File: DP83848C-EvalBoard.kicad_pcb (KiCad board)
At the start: 4 copper layers, 165 parts, among them J1 Conn_02x08_Odd_Even, J10 RJ45_LED_Shielded, J11 USB_C_Receptacle_USB2.0, J12 Conn_02x05_Odd_Even, J2 Conn_02x08_Odd_Even, J3 Conn_02x04_Odd_Even, J4 Conn_01x04, J5 Conn_01x04, J6 Conn_02x04_Odd_Even, J7 Conn_02x04_Odd_Even, J8 Conn_02x04_Odd_Even, J9 Conn_01x02, Q1 AO3401A, Q2 AO3400A, Q3 AO3401A, SW1 SW_Push, T1 H1102NL, U1 AMS1117-3.3, U2 DP83848C, U3 STM32F407VGTx, U4 USBLC6-2SC6, X1 50MHz, Y1 25MHz

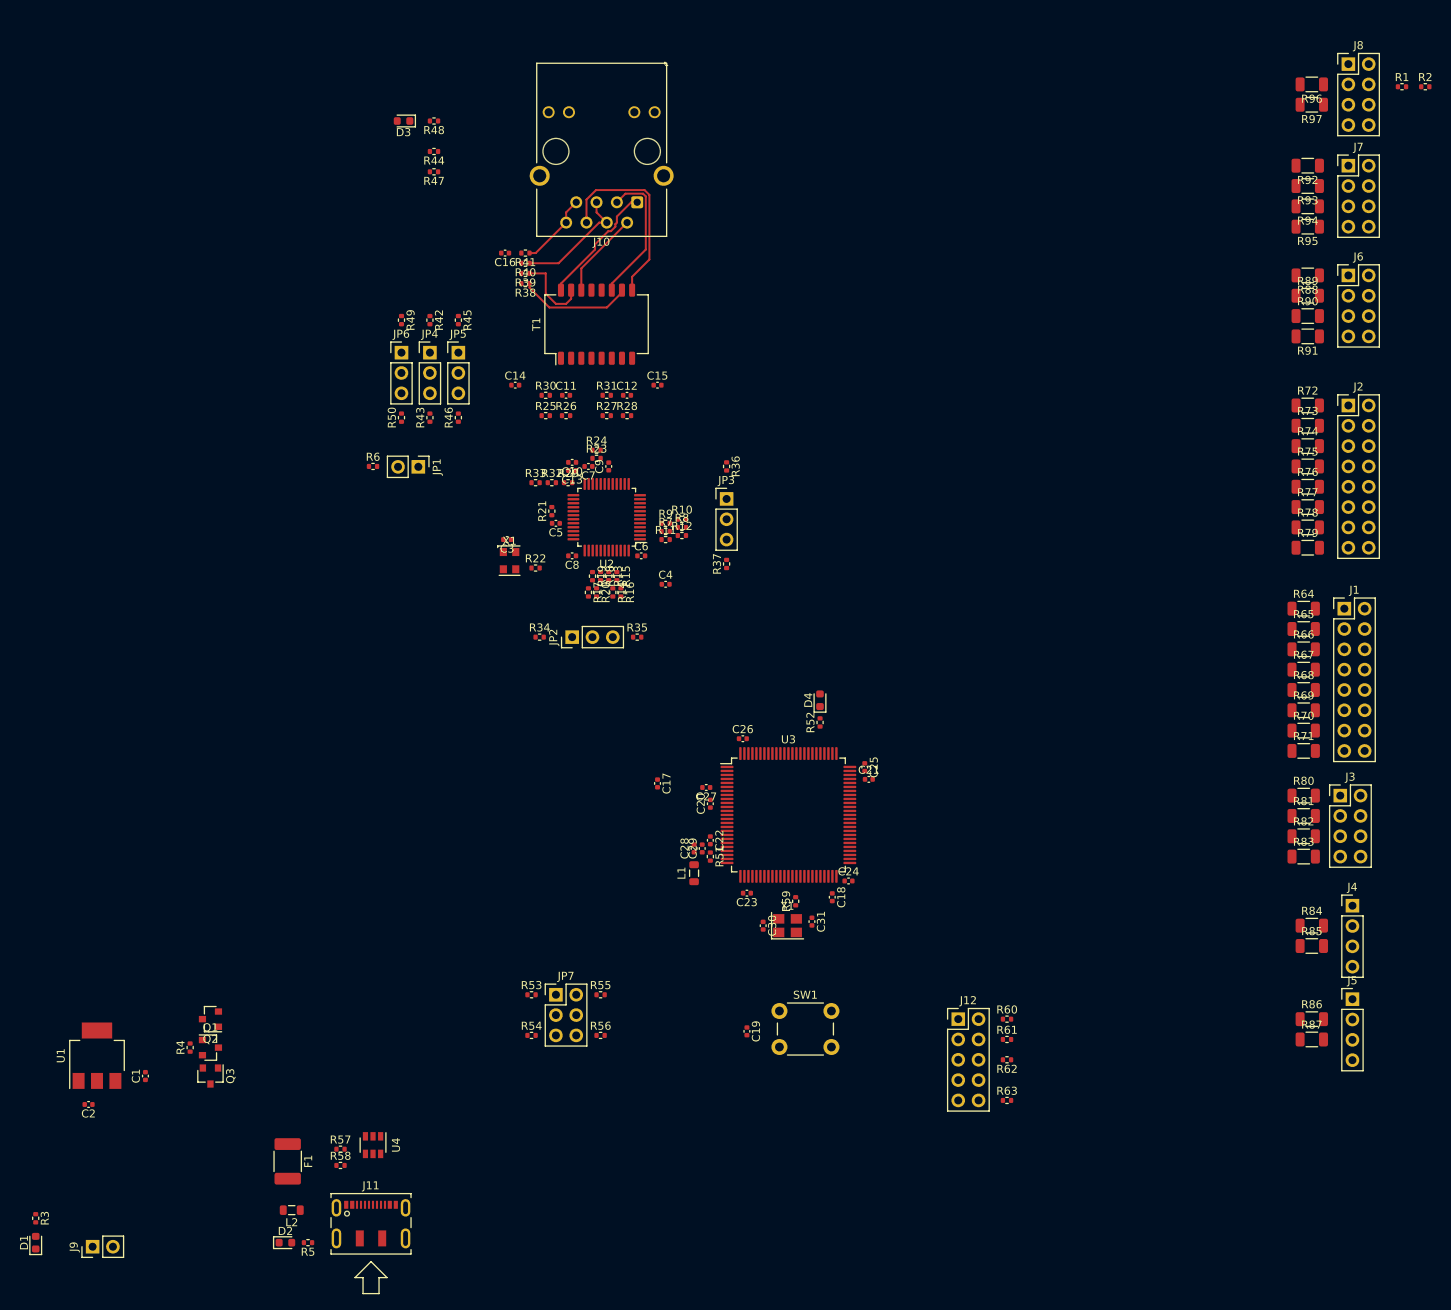
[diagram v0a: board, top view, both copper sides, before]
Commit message: Test...
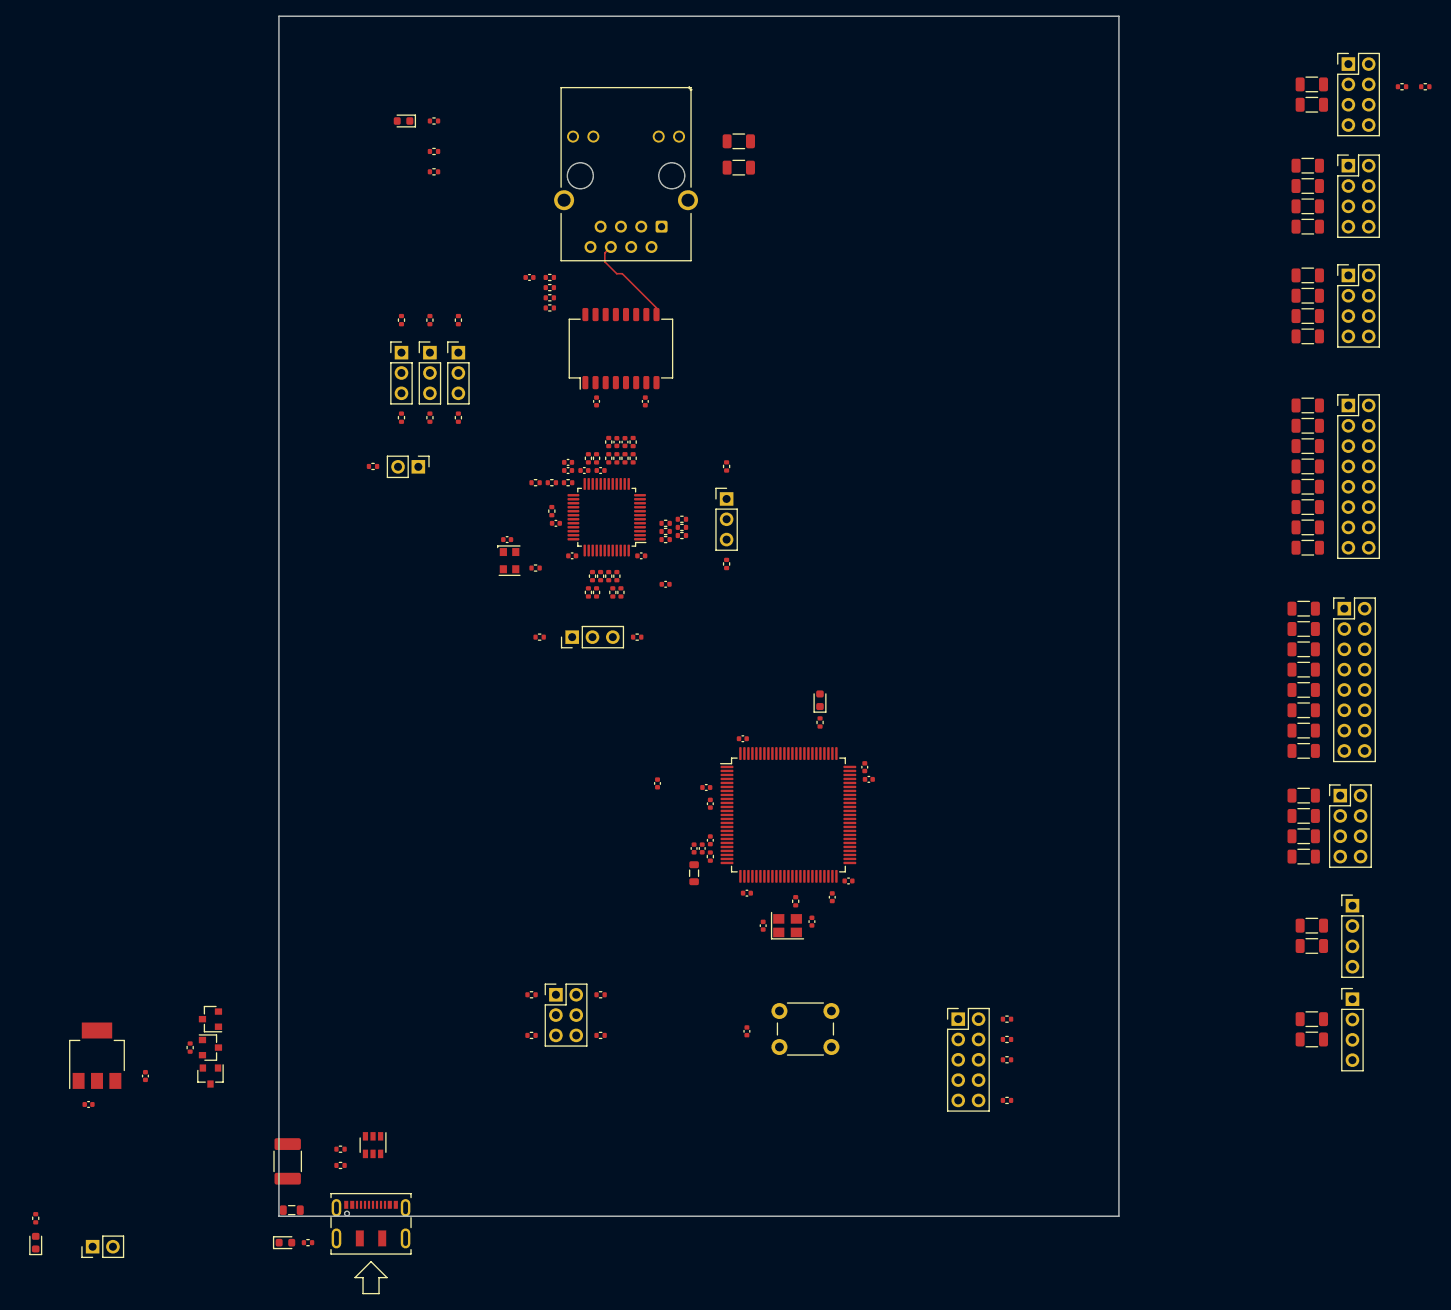
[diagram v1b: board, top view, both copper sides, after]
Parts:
- added R98: 0, Resistor_SMD:R_1206_3216Metric, F.Cu at (157.5, 40.6)
- added R99: 0, Resistor_SMD:R_1206_3216Metric, F.Cu at (157.5, 43.9)
- moved C14 10.4 mm to (139.7, 73.2), turned to 270 degrees
- moved R30 9.80 mm to (141.2, 78.2), turned to 270 degrees
- moved R25 9.51 mm to (141.2, 80.3), turned to 90 degrees
- moved C11 8.63 mm to (142.2, 78.2), turned to 90 degrees
- moved R26 8.29 mm to (142.2, 80.3), turned to 270 degrees
- moved R31 6.71 mm to (144.3, 78.2), turned to 270 degrees
- moved C12 5.85 mm to (143.3, 78.2), turned to 90 degrees
- moved R27 5.80 mm to (143.3, 80.3), turned to 90 degrees
- moved R28 5.39 mm to (144.3, 80.3), turned to 270 degrees
- moved C16 4.31 mm to (131.3, 57.7)
- moved J10 4.31 mm to (147.8, 51.3)
- moved R38 4.31 mm to (133.9, 61.5)
- moved R39 4.31 mm to (133.9, 60.2)
- moved R41 4.31 mm to (133.9, 57.7)
- moved T1 4.31 mm to (142.7, 66.5)
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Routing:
- net /PHY/RX+: track 17.7 -> 0.00 mm
- net /PHY/TX+: track 15.6 -> 0.00 mm
- net Net-(J10-Pad4): track 14.8 -> 0.00 mm
- net /PHY/RXC: track 14.2 -> 0.00 mm
- net /PHY/RX-: track 24.3 -> 11.8 mm
- net /PHY/TX-: track 10.8 -> 0.00 mm
- net /PHY/TXC: track 9.61 -> 0.00 mm
- net Net-(J10-Pad7): track 9.22 -> 0.00 mm
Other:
- board outline added: 105 x 150 mm
- net class Default: trace_width 0.25 -> 0.2; via_dia 0.8 -> 0.6; via_drill 0.4 -> 0.3
